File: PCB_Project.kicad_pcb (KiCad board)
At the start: 2 copper layers, 60 x 44.3 mm, 10 parts, among them SW1 SW_Push, SW2 SW_Push, SW3 SW_Push, U1 XIAO-RP2040-DIP

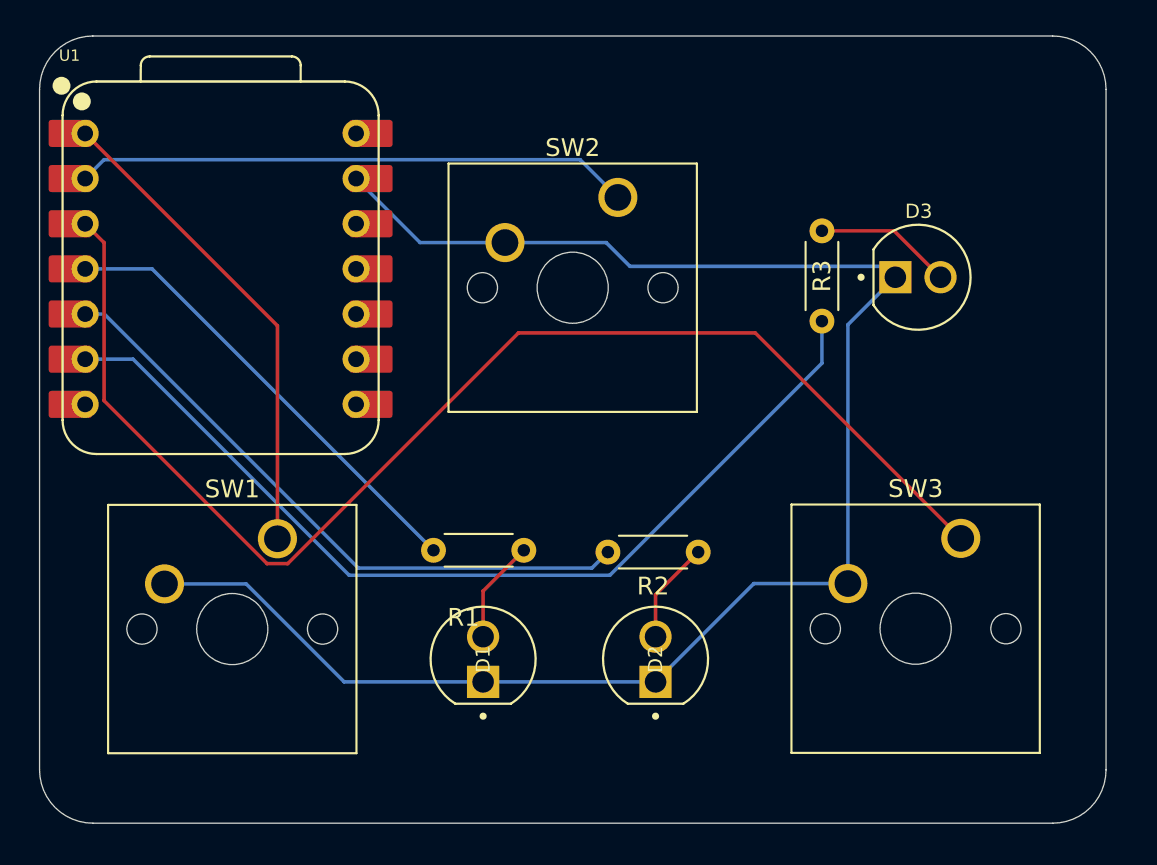
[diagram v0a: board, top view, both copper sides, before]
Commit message: Add files via upload
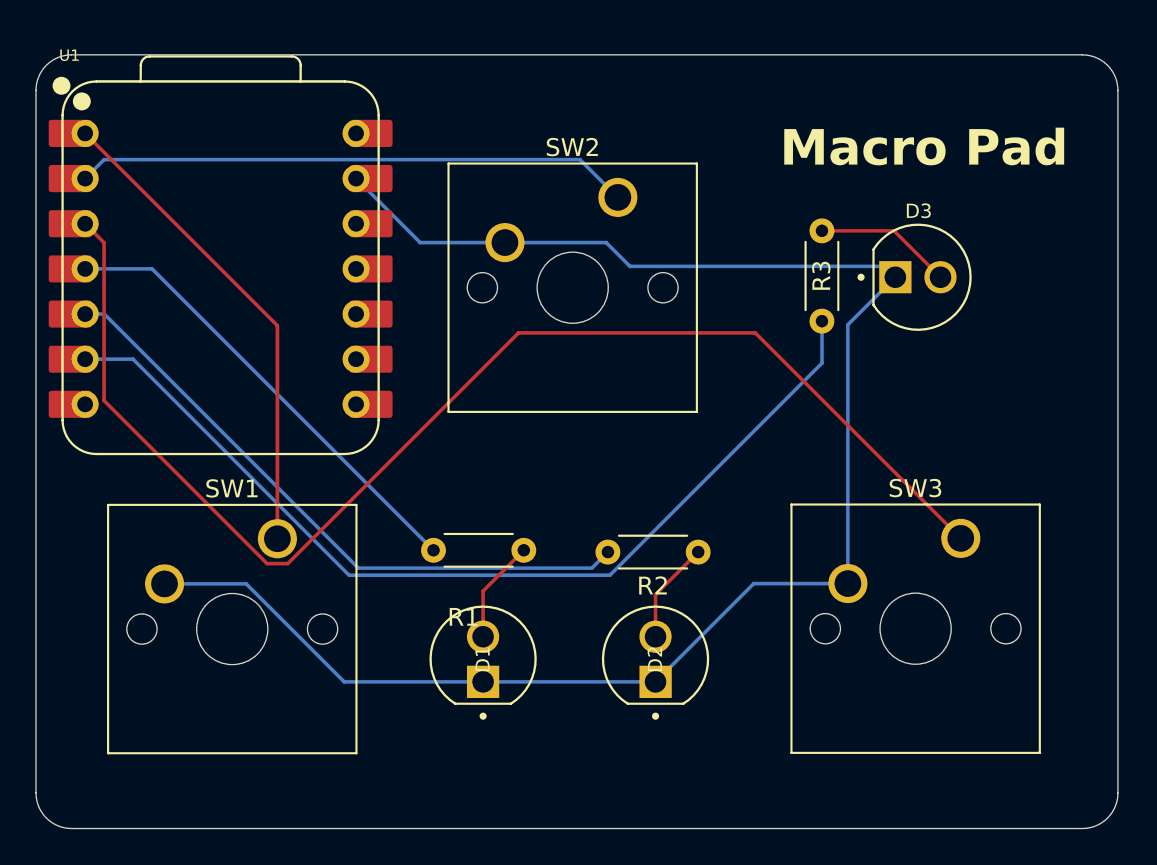
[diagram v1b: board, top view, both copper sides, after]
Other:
- board size 60 x 44.3 mm -> 60.9 x 43.5 mm
- board text added: "Macro Pad"
